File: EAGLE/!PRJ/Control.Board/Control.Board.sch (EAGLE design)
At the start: 55 parts, among them J1 AVR_SPI_PROG_3X2PTH, U1.X LTV817LTV817S, U1.Y LTV817LTV817S, U1.Z LTV817LTV817S, U2.X LTV817LTV817S, U2.Y LTV817LTV817S, U2.Z LTV817LTV817S

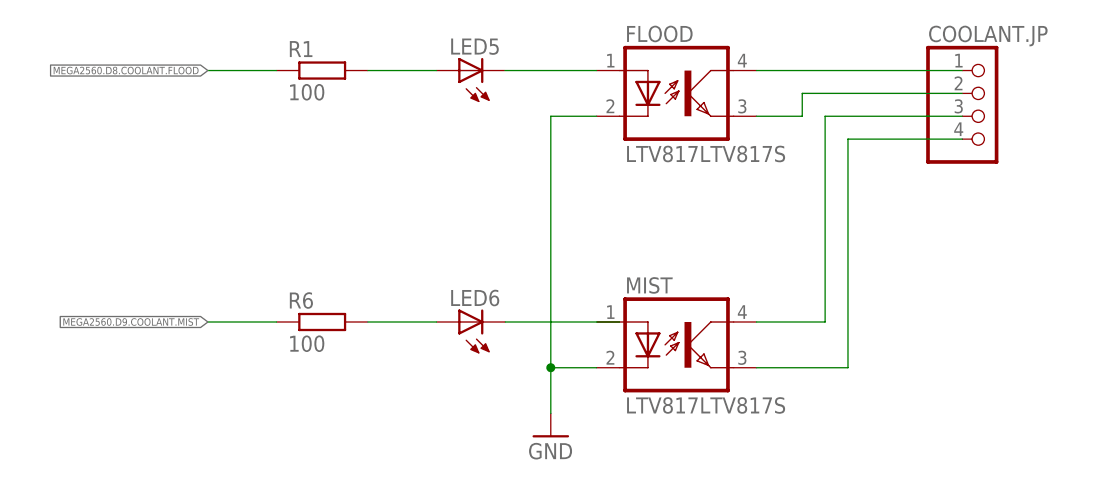
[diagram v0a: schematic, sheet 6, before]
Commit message: 20180511
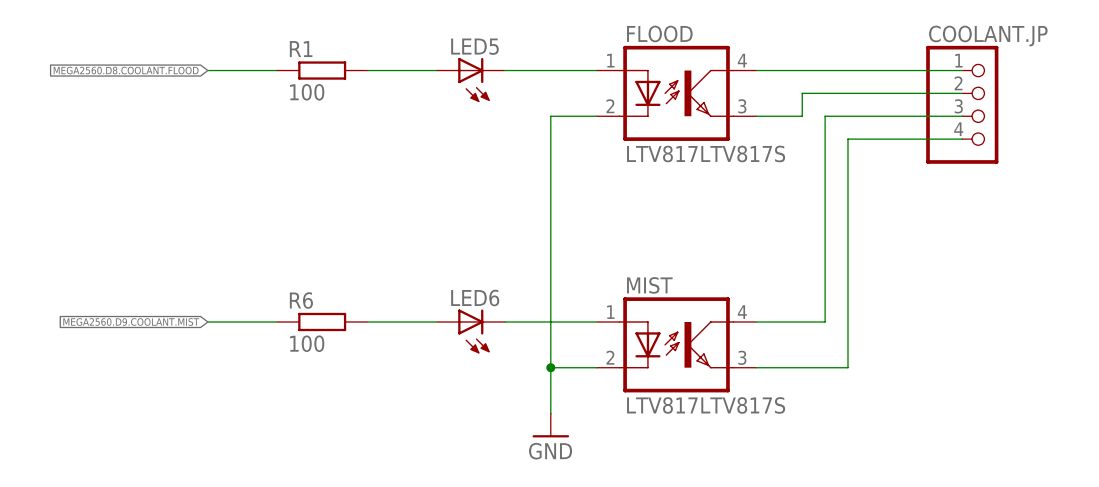
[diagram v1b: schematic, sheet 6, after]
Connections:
- net N$37: now also MIST.A
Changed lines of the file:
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@@
 <segment>
 <pinref part="LED6" gate="G$1" pin="C"/>
-<wire x1="58.42" y1="45.72" x2="71.12" y2="45.72" width="0.1524" layer="91"/>
+<pinref part="MIST" gate="G$1" pin="A"/>
+<wire x1="58.42" y1="45.72" x2="68.58" y2="45.72" width="0.1524" layer="91"/>
 </segment>
 </net>

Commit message: 20180511
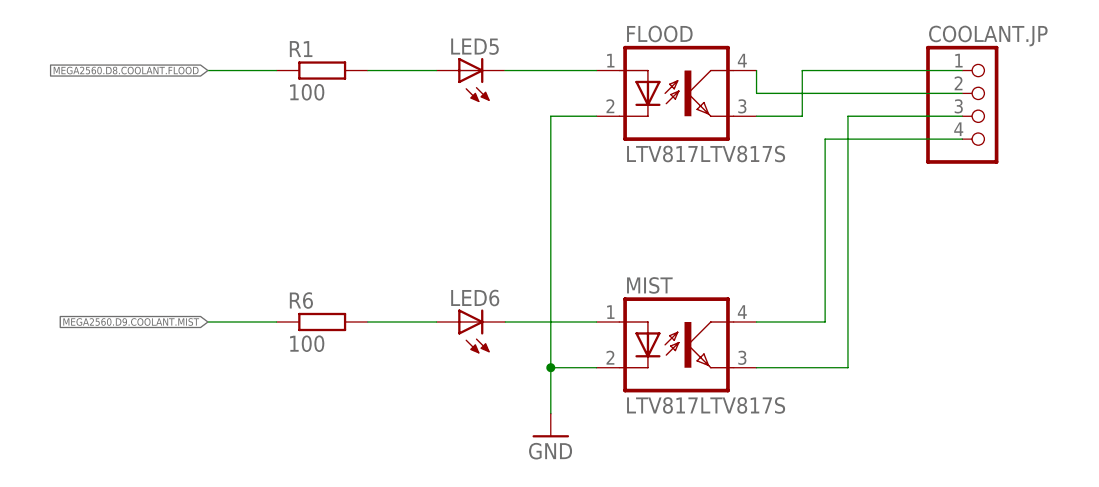
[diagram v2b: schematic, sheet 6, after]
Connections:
- net N$13: now also COOLANT.JP.2; no longer COOLANT.JP.1
- net N$15: now also COOLANT.JP.4; no longer COOLANT.JP.3
- net N$6: now also COOLANT.JP.1; no longer COOLANT.JP.2
- net N$9: now also COOLANT.JP.3; no longer COOLANT.JP.4
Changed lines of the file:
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@@
 <pinref part="FLOOD" gate="G$1" pin="EMIT"/>
 <wire x1="86.36" y1="68.58" x2="91.44" y2="68.58" width="0.1524" layer="91"/>
-<wire x1="91.44" y1="68.58" x2="91.44" y2="71.12" width="0.1524" layer="91"/>
-<pinref part="COOLANT.JP" gate="A" pin="2"/>
-<wire x1="91.44" y1="71.12" x2="109.22" y2="71.12" width="0.1524" layer="91"/>
+<pinref part="COOLANT.JP" gate="A" pin="1"/>
+<wire x1="91.44" y1="68.58" x2="91.44" y2="73.66" width="0.1524" layer="91"/>
+<wire x1="91.44" y1="73.66" x2="109.22" y2="73.66" width="0.1524" layer="91"/>
 </segment>
 </net>
@@
 <pinref part="MIST" gate="G$1" pin="EMIT"/>
 <wire x1="86.36" y1="40.64" x2="96.52" y2="40.64" width="0.1524" layer="91"/>
-<wire x1="96.52" y1="40.64" x2="96.52" y2="66.04" width="0.1524" layer="91"/>
-<pinref part="COOLANT.JP" gate="A" pin="4"/>
-<wire x1="96.52" y1="66.04" x2="109.22" y2="66.04" width="0.1524" layer="91"/>
+<pinref part="COOLANT.JP" gate="A" pin="3"/>
+<wire x1="96.52" y1="40.64" x2="96.52" y2="68.58" width="0.1524" layer="91"/>
+<wire x1="96.52" y1="68.58" x2="109.22" y2="68.58" width="0.1524" layer="91"/>
 </segment>
 </net>
@@
 </segment>
 </net>
-<net name="N$13" class="0">
-<segment>
-<pinref part="FLOOD" gate="G$1" pin="COL"/>
-<pinref part="COOLANT.JP" gate="A" pin="1"/>
-<wire x1="86.36" y1="73.66" x2="109.22" y2="73.66" width="0.1524" layer="91"/>
-</segment>
-</net>
 <net name="N$15" class="0">
 <segment>
-<pinref part="COOLANT.JP" gate="A" pin="3"/>
-<wire x1="109.22" y1="68.58" x2="93.98" y2="68.58" width="0.1524" layer="91"/>
-<wire x1="93.98" y1="68.58" x2="93.98" y2="45.72" width="0.1524" layer="91"/>
 <pinref part="MIST" gate="G$1" pin="COL"/>
 <wire x1="93.98" y1="45.72" x2="86.36" y2="45.72" width="0.1524" layer="91"/>
+<pinref part="COOLANT.JP" gate="A" pin="4"/>
+<wire x1="93.98" y1="45.72" x2="93.98" y2="66.04" width="0.1524" layer="91"/>
+<wire x1="93.98" y1="66.04" x2="109.22" y2="66.04" width="0.1524" layer="91"/>
 </segment>
 </net>
@@
 </segment>
 </net>
+<net name="N$13" class="0">
+<segment>
+<pinref part="FLOOD" gate="G$1" pin="COL"/>
+<pinref part="COOLANT.JP" gate="A" pin="2"/>
+<wire x1="86.36" y1="73.66" x2="86.36" y2="71.12" width="0.1524" layer="91"/>
+<wire x1="86.36" y1="71.12" x2="109.22" y2="71.12" width="0.1524" layer="91"/>
+</segment>
+</net>
